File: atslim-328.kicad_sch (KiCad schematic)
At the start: 13 parts, among them J1 UPDI, J2 RESET, J6 GPIO, U1 ATmega3208-M

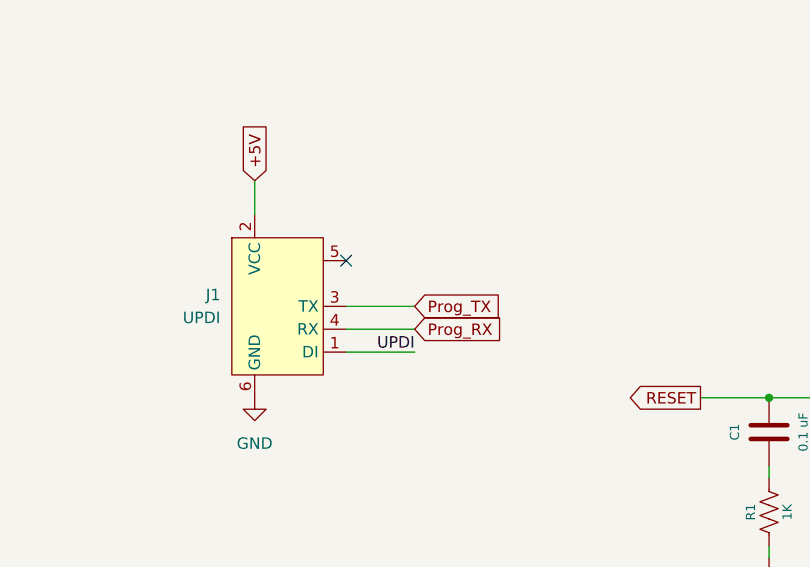
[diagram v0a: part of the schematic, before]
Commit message: Fucked up UPDI... of course
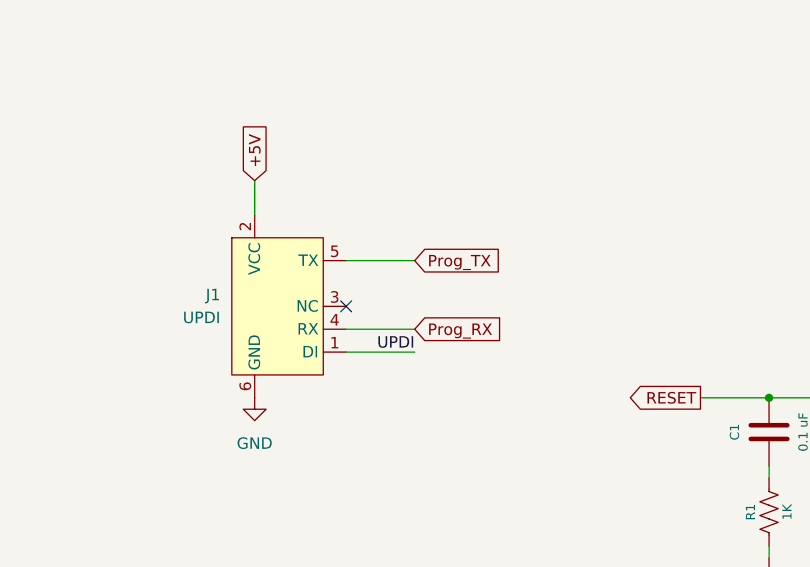
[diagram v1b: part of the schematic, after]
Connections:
- net Prog_TX: now also J1.5 (TX); no longer J1.3 (TX)
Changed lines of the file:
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@@
+	)
+	(no_connect
+		(at 87.63 88.9)
 	)
 	(no_connect
@@
 	)
 	(no_connect
-		(at 87.63 83.82)
-	)
-	(no_connect
 		(at 149.86 133.35)
 	)
@@
 	(wire
 		(pts
+			(xy 87.63 83.82) (xy 95.25 83.82)
+		)
+		(stroke
+			(width 0)
+			(type default)
+		)
+	)
+	(wire
+		(pts
 			(xy 237.49 53.34) (xy 248.92 53.34)
 		)
@@
 		(pts
 			(xy 237.49 45.72) (xy 248.92 45.72)
-		)
-		(stroke
-			(width 0)
-			(type default)
-		)
-	)
-	(wire
-		(pts
-			(xy 87.63 88.9) (xy 95.25 88.9)
 		)
 		(stroke
@@
 		)
 	)
-	(global_label "+5V"
+	(global_label "Prog_TX"
 		(shape input)
-		(at 77.47 74.93 90)
+		(at 95.25 83.82 0)
 		(fields_autoplaced yes)
 		(effects
@@
 		)
 		(property "Intersheetrefs" "${INTERSHEET_REFS}"
-			(at 77.47 68.0743 90)
+			(at 106.0366 83.82 0)
 			(effects
 				(font
@@
 		)
 	)
-	(global_label "Prog_TX"
+	(global_label "+5V"
 		(shape input)
-		(at 95.25 88.9 0)
+		(at 77.47 74.93 90)
 		(fields_autoplaced yes)
 		(effects
@@
 		)
 		(property "Intersheetrefs" "${INTERSHEET_REFS}"
-			(at 106.0366 88.9 0)
+			(at 77.47 68.0743 90)
 			(effects
 				(font
